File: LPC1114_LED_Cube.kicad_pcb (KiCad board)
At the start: 2 copper layers, 100 x 100 mm, 80 parts, among them Q201 BSS138, Q202 BSS138, Q203 BSS138, Q204 BSS138, Q205 IRLML6402TRPBF, Q206 IRLML6402TRPBF, Q207 IRLML6402TRPBF, Q208 IRLML6402TRPBF, Q209 BSS138, Q210 BSS138, Q211 BSS138, Q212 BSS138, Q213 IRLML6402TRPBF, Q214 IRLML6402TRPBF, Q215 IRLML6402TRPBF, Q216 IRLML6402TRPBF, Y101 12MHZ, Y102 12MHZ

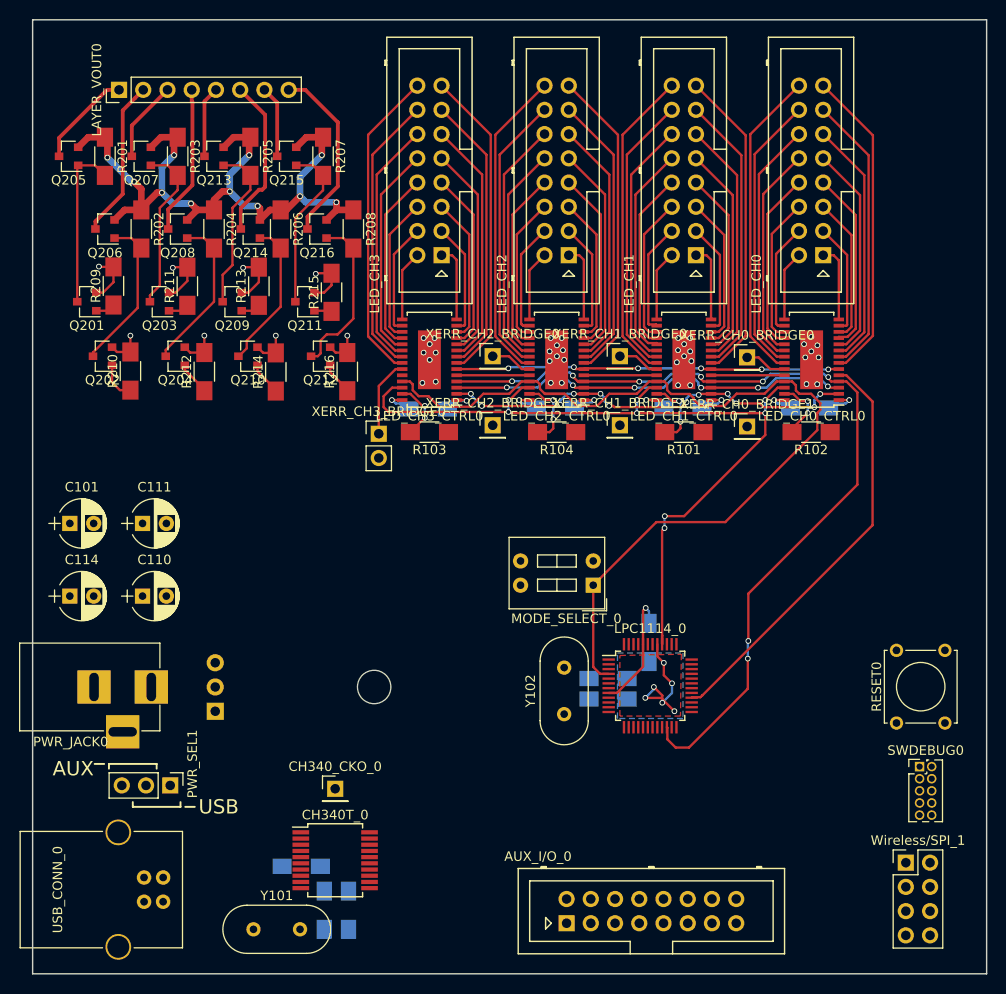
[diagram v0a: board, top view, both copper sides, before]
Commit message: more PCB layout
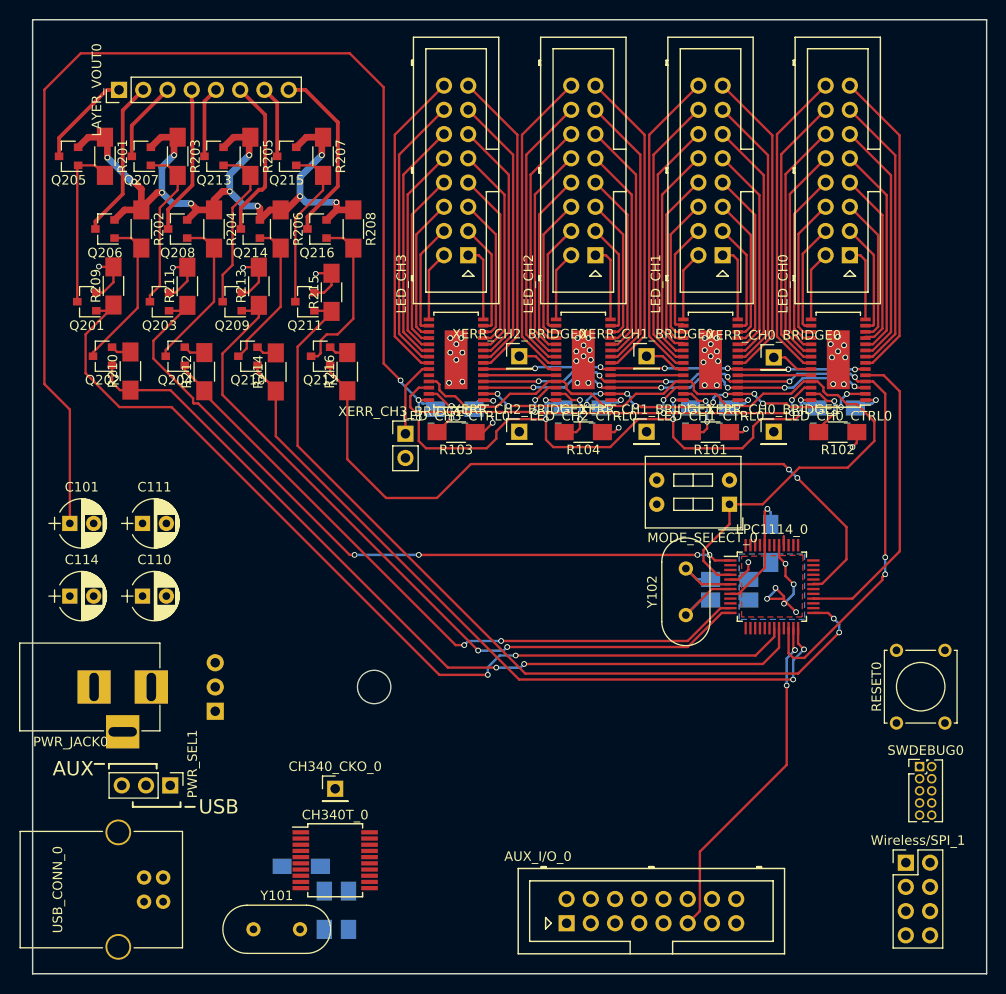
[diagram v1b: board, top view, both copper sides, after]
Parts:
- moved MODE_SELECT_0 16.6 mm to (158.0, 95.8)
- moved C107 16.4 mm to (158.1, 103.7)
- moved LPC1114_0 16.4 mm to (162.5, 104.4)
- moved C104 16.4 mm to (162.4, 99.9)
- moved C106 16.4 mm to (158.1, 105.8)
- moved Y102 16.4 mm to (153.5, 107.4)
- moved XERR_CH1_BRIDGE1 2.87 mm to (149.4, 88.2)
- moved XERR_CH2_BRIDGE1 2.87 mm to (136.0, 88.2)
- moved XERR_CH0_BRIDGE1 2.85 mm to (162.7, 88.2)
- moved C109 2.79 mm to (156.0, 85.7)
- moved C113 2.79 mm to (142.6, 85.7)
- moved LED_CH1 2.79 mm to (157.3, 69.7)
- moved LED_CH1_CTRL0 2.79 mm to (156.1, 80.6)
- moved LED_CH2 2.79 mm to (144.0, 69.7)
- moved LED_CH3_CTRL0 2.79 mm to (129.4, 80.6)
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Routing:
- net V3: track 25.0 -> 204.6 mm, vias 5 -> 10
- net LAYER_0_ON: track 2.04 -> 98.7 mm, vias 0 -> 2
- net LAYER_6_ON: track 1.82 -> 89.9 mm, vias 0 -> 2
- net LAYER_1_ON: track 4.05 -> 87.0 mm, vias 0 -> 2
- net LAYER_4_ON: track 2.03 -> 79.0 mm, vias 0 -> 2
- net LAYER_2_ON: track 2.16 -> 78.7 mm, vias 0 -> 4
- net LAYER_5_ON: track 3.50 -> 79.1 mm, vias 0 -> 2
- net LAYER_7_ON: track 3.41 -> 76.8 mm, vias 0 -> 2
- net LAYER_3_ON: track 3.52 -> 71.5 mm, vias 0 -> 2
- net PIO0_7: track 0.00 -> 35.7 mm, vias 0 -> 2
- net DCPRG: track 86.6 -> 56.7 mm, vias 8 -> 6
- net LED_DATA_SCK: track 94.0 -> 81.5 mm
- net LED_SIN: track 44.1 -> 32.2 mm
- net ISP_ENTRY: track 98.4 -> 88.8 mm
- net Net-(C106-Pad1): track 0.00 -> 9.05 mm
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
